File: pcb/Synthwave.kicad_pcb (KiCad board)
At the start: 2 copper layers, 68.8 x 136.6 mm, 66 parts, among them J1 Conn_01x01_Pin, J2 Conn_01x01_Pin, J3 ADC1, J4 ADC2, J5 ADC3, J6 ADC4, P1 MINI-360, P2 MINI-360, Q1 TIP120, Q10 TIP120, Q2 TIP120, Q3 TIP120, Q4 TIP120, Q5 TIP120, Q6 TIP120, Q7 TIP120, Q8 TIP120, Q9 TIP120, U1 Heltec_HTIT-WB32v3, U2 L9110

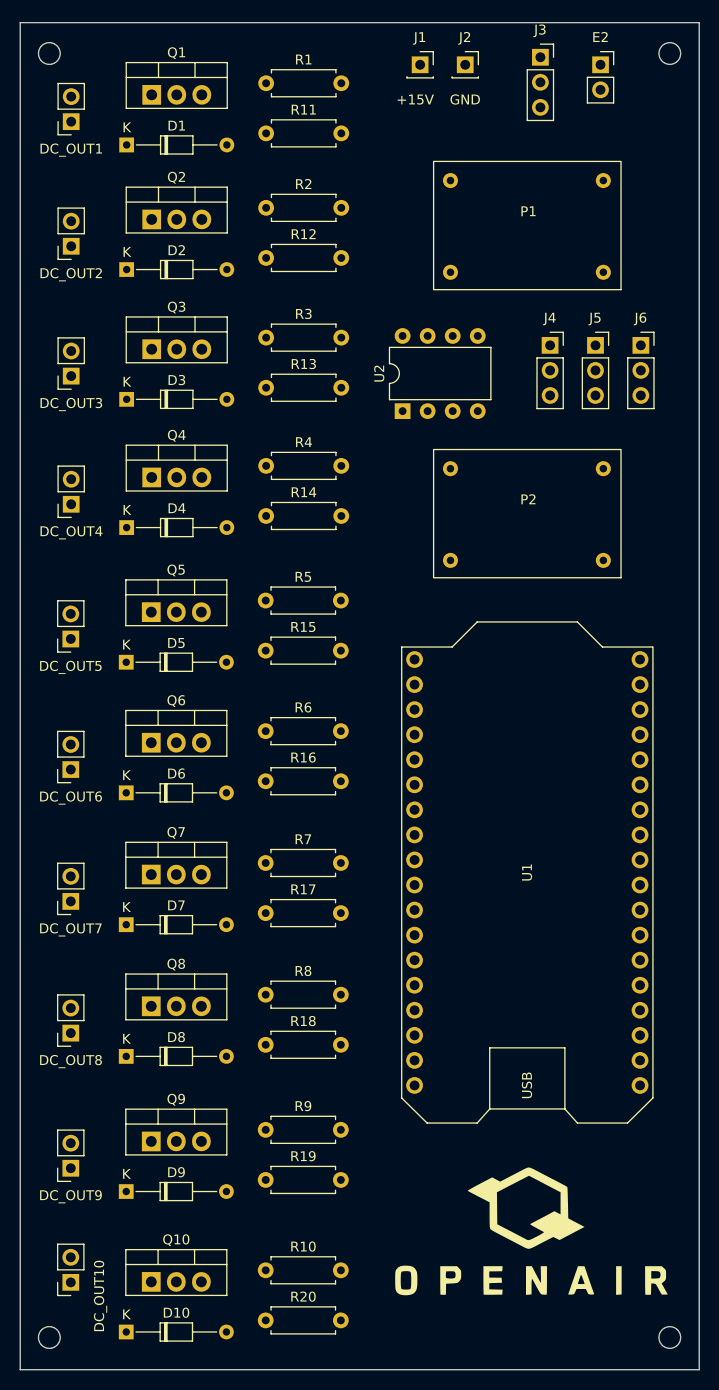
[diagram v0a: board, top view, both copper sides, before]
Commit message: Update and upgrades
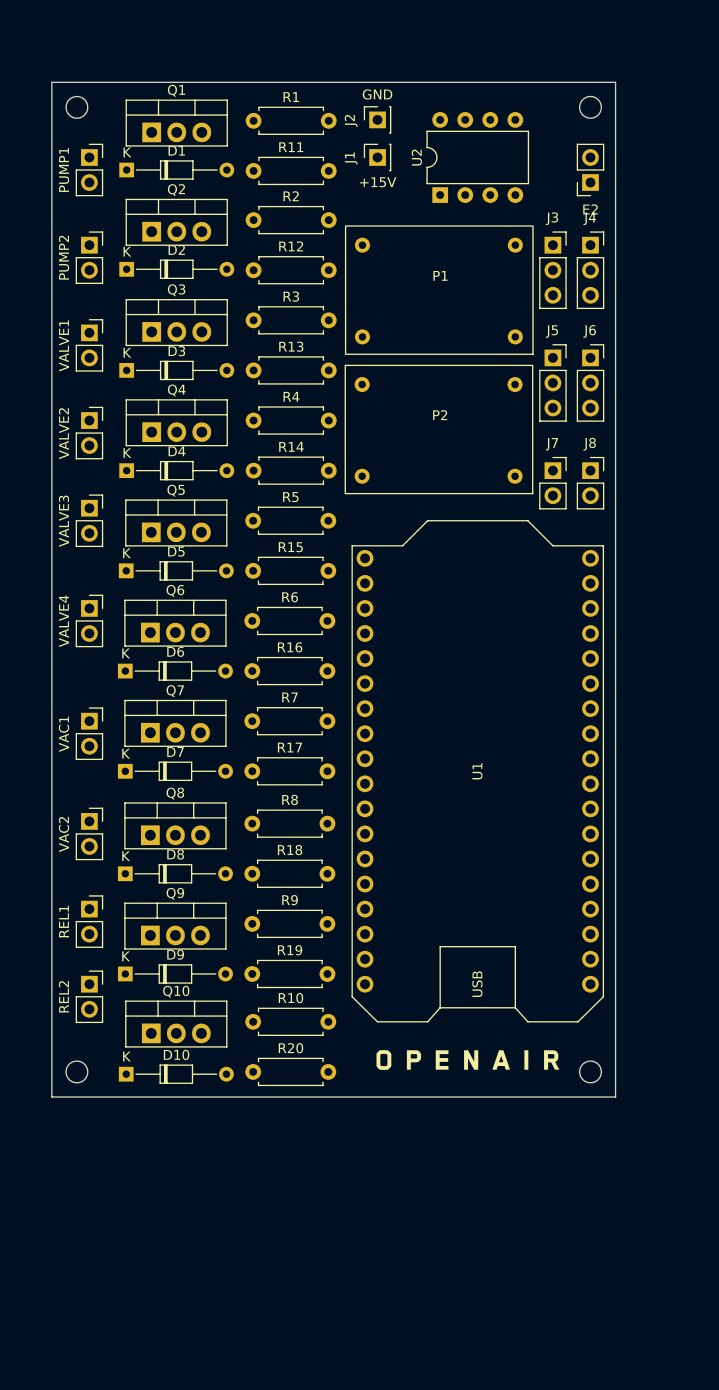
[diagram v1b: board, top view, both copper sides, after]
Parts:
- removed DC_OUT1, DC_OUT10, DC_OUT2, DC_OUT3, DC_OUT4, DC_OUT5, DC_OUT6, DC_OUT7, DC_OUT8, DC_OUT9: GND, Connector_PinSocket_2.54mm:PinSocket_1x02_P2.54mm_Vertical
- removed the G*** at (65.1, 136.6)
- added G***: LOGO, Untitled, F.Cu at (58.4, 118.1)
- added J7: RX, Connector_PinSocket_2.54mm:PinSocket_1x02_P2.54mm_Vertical, F.Cu at (67.3, 58.4)
- added J8: RX, Connector_PinSocket_2.54mm:PinSocket_1x02_P2.54mm_Vertical, F.Cu at (71.1, 58.4)
- added PUMP1: GND, Connector_PinSocket_2.54mm:PinSocket_1x02_P2.54mm_Vertical, F.Cu at (20.3, 26.7)
- added PUMP2: GND, Connector_PinSocket_2.54mm:PinSocket_1x02_P2.54mm_Vertical, F.Cu at (20.3, 35.6)
- added REL1: GND, Connector_PinSocket_2.54mm:PinSocket_1x02_P2.54mm_Vertical, F.Cu at (20.3, 102.9)
- added REL2: GND, Connector_PinSocket_2.54mm:PinSocket_1x02_P2.54mm_Vertical, F.Cu at (20.3, 110.5)
- added VAC1: GND, Connector_PinSocket_2.54mm:PinSocket_1x02_P2.54mm_Vertical, F.Cu at (20.3, 83.8)
- added VAC2: GND, Connector_PinSocket_2.54mm:PinSocket_1x02_P2.54mm_Vertical, F.Cu at (20.3, 94.0)
- added VALVE1: GND, Connector_PinSocket_2.54mm:PinSocket_1x02_P2.54mm_Vertical, F.Cu at (20.3, 44.5)
- added VALVE2: GND, Connector_PinSocket_2.54mm:PinSocket_1x02_P2.54mm_Vertical, F.Cu at (20.3, 53.3)
- added VALVE3: GND, Connector_PinSocket_2.54mm:PinSocket_1x02_P2.54mm_Vertical, F.Cu at (20.3, 62.2)
- added VALVE4: GND, Connector_PinSocket_2.54mm:PinSocket_1x02_P2.54mm_Vertical, F.Cu at (20.3, 72.4)
- moved H3 28.1 mm to (71.1, 119.4)
- moved H2 27.1 mm to (19.1, 119.4)
- moved D10 26.1 mm to (24.1, 119.6)
- moved R10 25.2 mm to (36.9, 114.3)
- moved R20 25.2 mm to (36.9, 119.4)
- moved Q10 25.2 mm to (26.6, 115.5)
- moved U2 22.2 mm to (55.9, 30.5)
- moved D9 22.1 mm to (24.0, 109.5)
- moved R19 20.9 mm to (36.8, 109.5)
- moved R9 20.9 mm to (36.8, 104.4)
- moved Q9 20.9 mm to (26.5, 105.5)
- moved J3 19.1 mm to (67.3, 35.6)
- moved D8 18.5 mm to (24.0, 99.3)
- moved R8 17.4 mm to (36.8, 94.2)
- moved R18 17.4 mm to (36.8, 99.3)
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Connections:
- U1 pad 12: unconnected-(U1-43_TX-Pad12) -> Net-(J7-Pin_1)
- U1 pad 13: unconnected-(U1-44_RX-Pad13) -> Net-(J7-Pin_2)
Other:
- board size 68.8 x 136.6 mm -> 57.1 x 102.9 mm
